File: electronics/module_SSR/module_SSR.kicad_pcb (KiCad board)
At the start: 2 copper layers, 50 x 25 mm, 8 parts

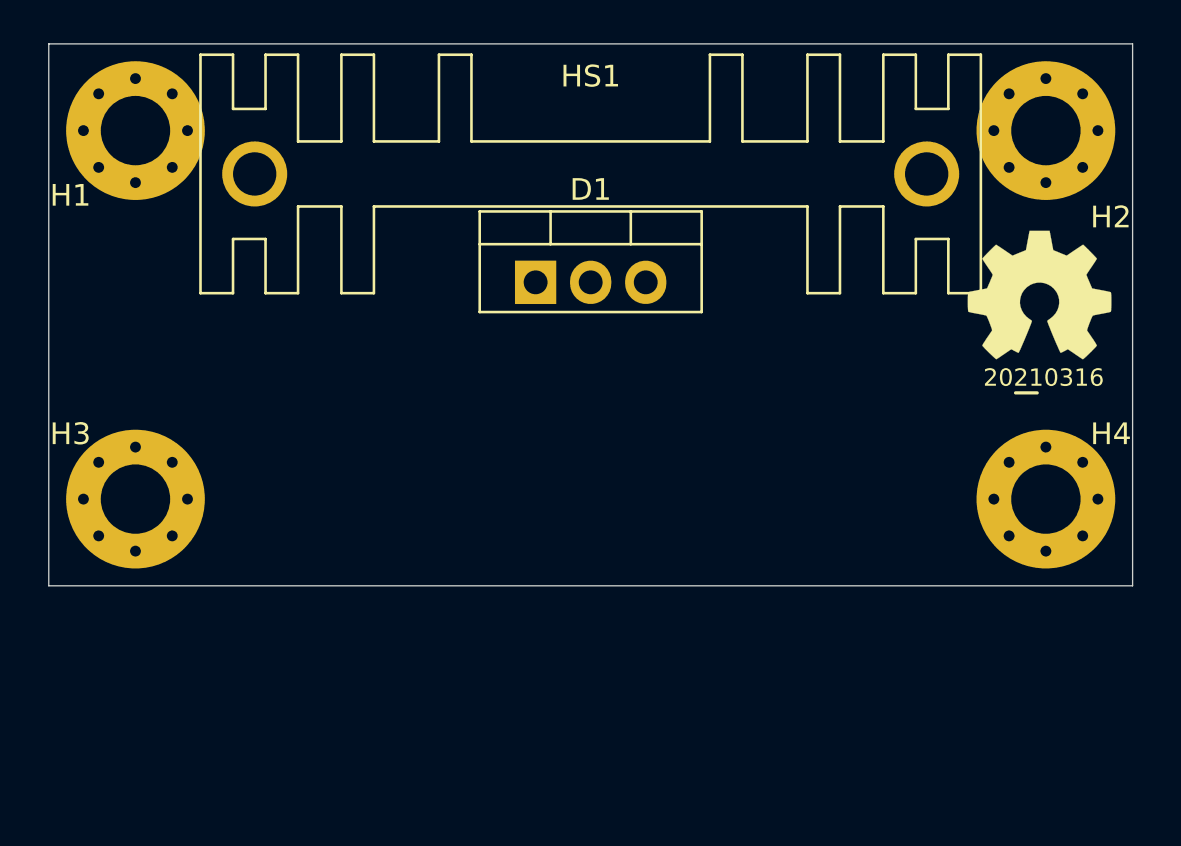
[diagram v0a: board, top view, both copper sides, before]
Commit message: schematic completed, placed and routed
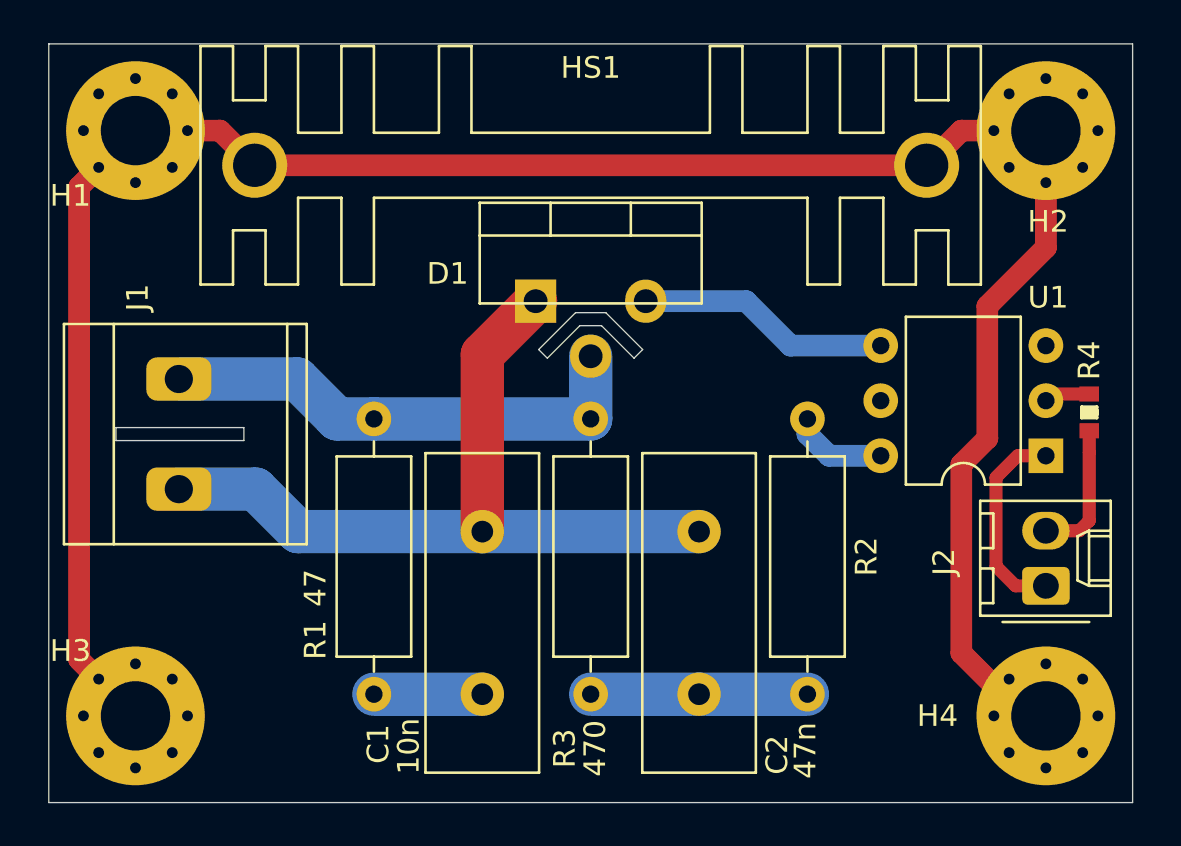
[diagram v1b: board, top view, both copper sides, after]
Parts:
- added C1: 10n, Capacitor_THT:C_Disc_D14.5mm_W5.0mm_P7.50mm, F.Cu at (150.0, 105.0)
- added C2: 47n, Capacitor_THT:C_Disc_D14.5mm_W5.0mm_P7.50mm, F.Cu at (160.0, 105.0)
- added J1: Conn_01x02, SquantorPhoenixContact:MKDS_2conn_508pitch_1711725, F.Cu at (136.0, 93.0)
- added J2: Conn_01x02, Connector_Molex:Molex_KK-254_AE-6410-02A_1x02_P2.54mm_Vertical, F.Cu at (176.0, 100.0)
- added R1: 47, Resistor_THT:R_Axial_DIN0309_L9.0mm_D3.2mm_P12.70mm_Horizontal, F.Cu at (145.0, 92.3)
- added R2: 330, Resistor_THT:R_Axial_DIN0309_L9.0mm_D3.2mm_P12.70mm_Horizontal, F.Cu at (165.0, 92.3)
- added R3: 470, Resistor_THT:R_Axial_DIN0309_L9.0mm_D3.2mm_P12.70mm_Horizontal, F.Cu at (155.0, 92.3)
- added R4: 1K, SquantorRcl:R_0603_hand, F.Cu at (178.0, 92.0)
- added U1: MOC3021M, Package_DIP:DIP-6_W7.62mm, F.Cu at (176.0, 94.0)
- D1: footprint Package_TO_SOT_THT:TO-220-3_Vertical -> SquantorIC:TO-220-3_Vertical_stagger
- N1, N2: moved to B.Cu
- moved N2 21.5 mm to (155.2, 80.2), turned to 180 degrees
- moved N1 20.3 mm to (155.8, 84.1), turned to 180 degrees
- moved H3 10.0 mm to (134.0, 106.0)
- moved H4 10.0 mm to (176.0, 106.0)
- moved D1 2.57 mm to (155.0, 85.6)
- moved HS1 0.40 mm to (155.0, 80.6)
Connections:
- D1 pad 1: Net-(D1-Pad1) -> /SWITCH
- D1 pad 2: Net-(D1-Pad2) -> /LIVE
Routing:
- net Earth: track 0.00 -> 103.3 mm
- net /SWITCH: track 0.00 -> 36.5 mm
- net /LIVE: track 0.00 -> 22.7 mm
- net Net-(D1-Pad3): track 0.00 -> 11.7 mm
- net Net-(C2-Pad1): track 0.00 -> 10.0 mm
- net /LED_A: track 0.00 -> 9.49 mm
- net /LED_C: track 0.00 -> 6.34 mm
- net Net-(C1-Pad1): track 0.00 -> 5.00 mm
- net Net-(R2-Pad1): track 0.00 -> 4.49 mm
- net Net-(R4-Pad1): track 0.00 -> 2.13 mm
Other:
- board size 50 x 25 mm -> 50 x 35 mm
